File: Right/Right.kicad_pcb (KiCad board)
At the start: 2 copper layers, 169.8 x 149.7 mm, 215 parts, among them SW0 SW_PUSH, SW1 SW_PUSH, SW10 SW_PUSH, SW100 SW_PUSH, SW1000 SW_Push_Dual_R, SW1001 SW_Push_Dual_R, SW1002 SW_Push_Dual_R, SW1003 SW_Push_Dual_R, SW1004 SW_Push_Dual_R, SW1005 SW_Push_Dual_R, SW101 SW_PUSH, SW102 SW_PUSH, SW103 SW_PUSH, SW104 SW_PUSH, SW105 SW_PUSH, SW106 SW_PUSH, SW11 SW_PUSH, SW110 SW_PUSH, SW111 SW_PUSH, SW112 SW_PUSH, SW113 SW_PUSH, SW114 SW_PUSH, SW115 SW_PUSH, SW116 SW_PUSH, SW12 SW_PUSH, SW13 SW_PUSH, SW14 SW_PUSH, SW15 SW_PUSH, SW2 SW_PUSH, SW20 SW_PUSH, SW21 SW_PUSH, SW22 SW_PUSH, SW23 SW_PUSH, SW24 SW_PUSH, SW25 SW_PUSH, SW3 SW_PUSH, SW30 SW_PUSH, SW31 SW_PUSH, SW32 SW_PUSH, SW33 SW_PUSH, SW34 SW_PUSH, SW35 SW_PUSH, SW36 SW_PUSH, SW37 SW_PUSH, SW38 SW_PUSH, SW39 SW_PUSH, SW4 SW_PUSH, SW40 SW_PUSH, SW41 SW_PUSH, SW42 SW_PUSH, SW43 SW_PUSH, SW44 SW_PUSH, SW45 SW_PUSH, SW5 SW_PUSH, SW50 SW_PUSH, SW51 SW_PUSH, SW52 SW_PUSH, SW53 SW_PUSH, SW54 SW_PUSH, SW60 SW_PUSH, SW61 SW_PUSH, SW62 SW_PUSH, SW63 SW_PUSH, SW64 SW_PUSH, SW65 SW_PUSH, SW66 SW_PUSH, SW70 SW_PUSH, SW71 SW_PUSH, SW72 SW_PUSH, SW73 SW_PUSH, SW74 SW_PUSH, SW75 SW_PUSH, SW76 SW_PUSH, SW77 SW_PUSH, SW80 SW_PUSH, SW81 SW_PUSH, SW82 SW_PUSH, SW83 SW_PUSH, SW84 SW_PUSH, SW85 SW_PUSH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

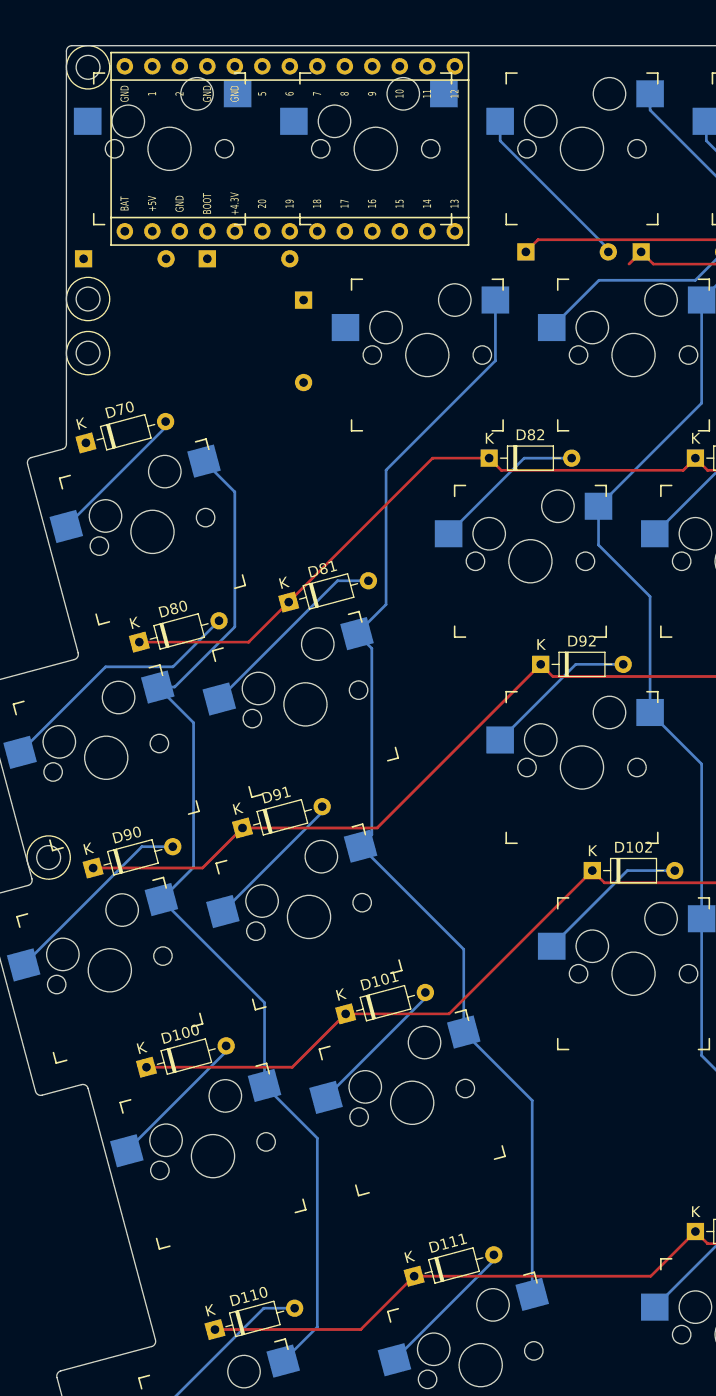
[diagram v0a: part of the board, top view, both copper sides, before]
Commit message: 途中
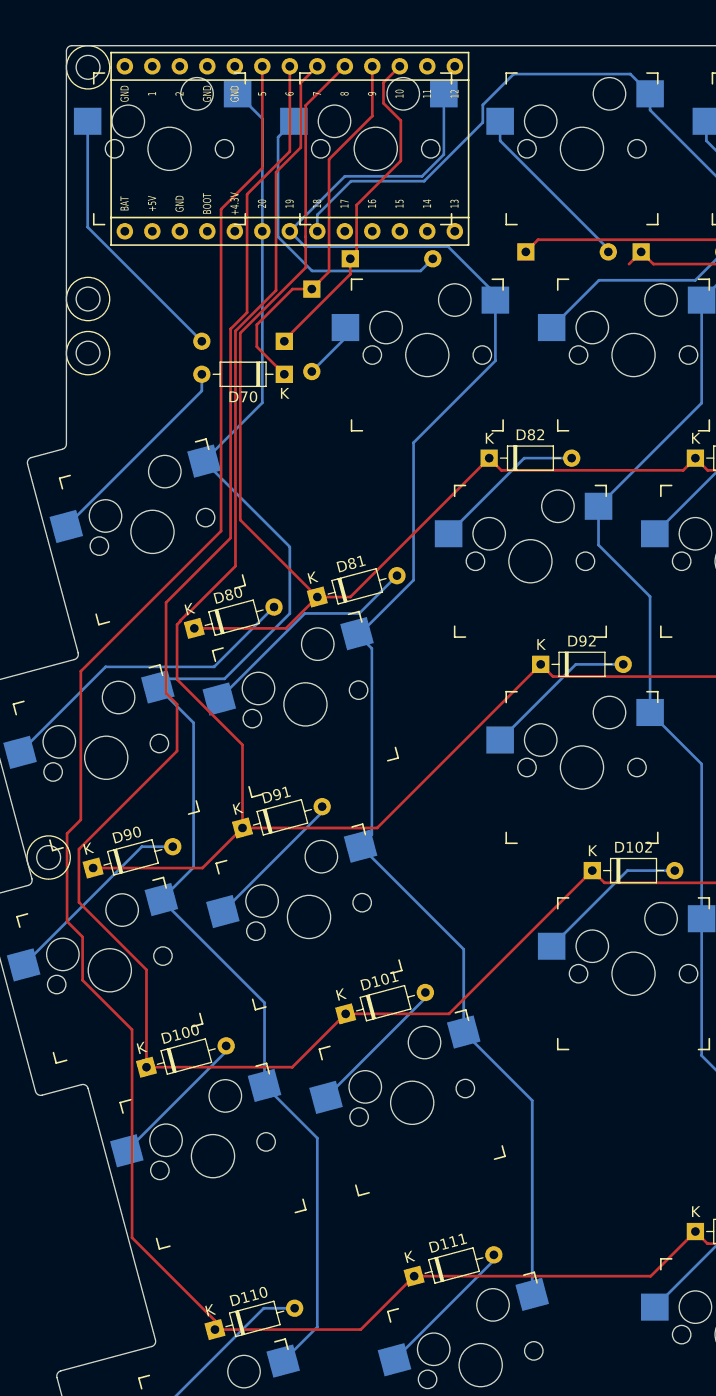
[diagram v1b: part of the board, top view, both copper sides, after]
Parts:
- moved D60 20.0 mm to (177.3, 17.8), turned to 180 degrees
- moved D70 19.4 mm to (177.3, 20.8), turned to 180 degrees
- moved D61 13.2 mm to (183.4, 10.2)
- moved D80 5.24 mm to (169.0, 44.3)
- moved D81 2.68 mm to (180.3, 41.4)
- moved D71 1.27 mm to (179.8, 13.0)
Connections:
- BPM1 pad 16: row0 -> row5
- BPM1 pad 17: row1 -> row4
- BPM1 pad 18: row2 -> row3
- BPM1 pad 19: row3 -> row2
- BPM1 pad 20: row4 -> row1
- BPM1 pad 21: row5 -> row0
- BPM2 pad 10: col10 -> row7
- BPM2 pad 11: col11 -> row6
- BPM2 pad 12: col12 -> led1
- BPM2 pad 13: col13 -> rowsys1
- BPM2 pad 14: rowsys1 -> col13
- BPM2 pad 15: led1 -> col12
- BPM2 pad 16: row6 -> col11
- BPM2 pad 17: row7 -> col10
- BPM2 pad 18: row8 -> col9
- BPM2 pad 19: row9 -> col8
- BPM2 pad 20: row10 -> col7
- BPM2 pad 21: row11 -> col6
- BPM2 pad 6: col6 -> row11
- BPM2 pad 7: col7 -> row10
- BPM2 pad 8: col8 -> row9
- BPM2 pad 9: col9 -> row8
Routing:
- net row11: track 145.4 -> 275.2 mm
- net row10: track 146.5 -> 250.4 mm
- net row9: track 139.9 -> 218.1 mm
- net row8: track 159.2 -> 209.5 mm
- net col7: track 105.0 -> 149.9 mm
- net col6: track 98.3 -> 141.9 mm
- net col8: track 126.2 -> 165.6 mm
- net row7: track 108.7 -> 143.6 mm
- net row6: track 100.9 -> 132.1 mm
- net Net-(D61-Pad2): track 0.00 -> 27.4 mm
- net Net-(D60-Pad2): track 0.00 -> 24.7 mm
- net Net-(D70-Pad2): track 13.5 -> 19.2 mm
- net Net-(D80-Pad2): track 23.4 -> 29.0 mm
- net Net-(D71-Pad2): track 0.00 -> 5.35 mm
- net Net-(D81-Pad2): track 18.3 -> 21.1 mm
